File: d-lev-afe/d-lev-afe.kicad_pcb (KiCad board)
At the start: 4 copper layers, 89 x 50 mm, 37 parts, among them J1 S8B-PH-SM4-TB, Q1 MMBT3904, Q2 MMBT3906, U1 74AHC04, U2 AP2112K-3.3, U3 SRV05-4

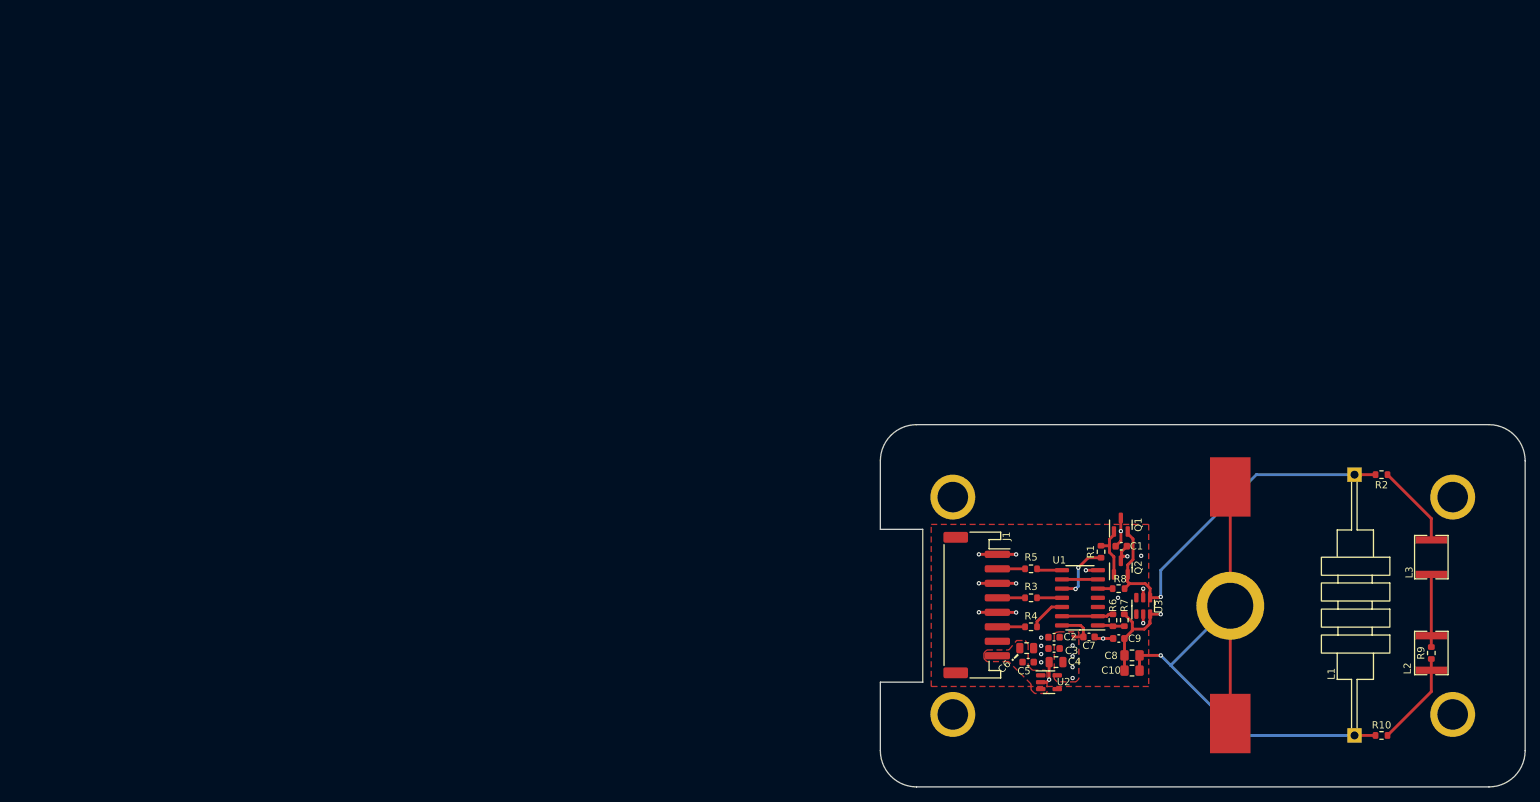
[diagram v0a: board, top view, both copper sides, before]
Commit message: Add JLC releases
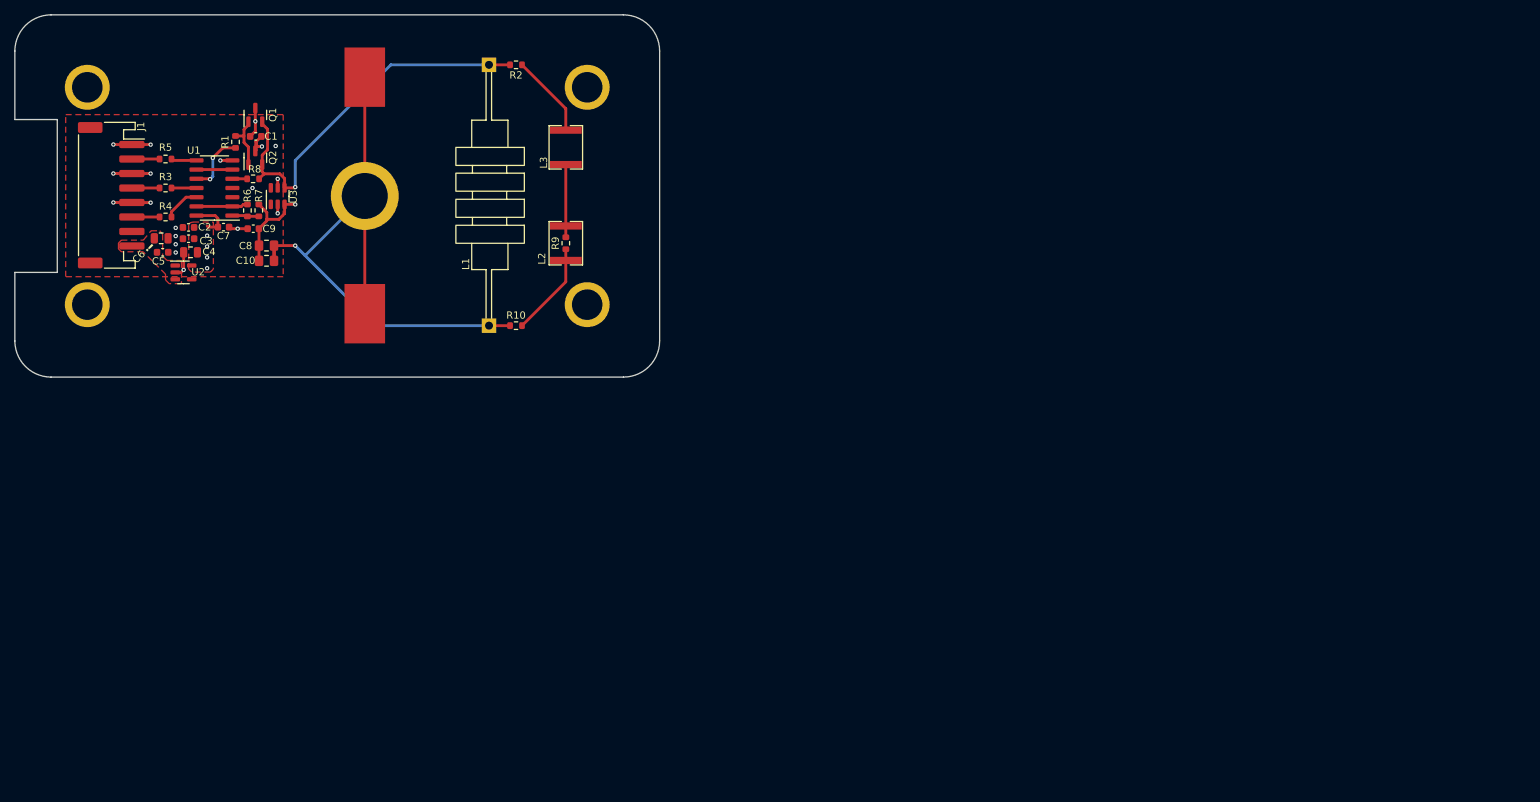
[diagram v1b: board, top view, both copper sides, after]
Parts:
- moved AE1 132.2 mm to (61.8, 25.9)
- moved AE2 132.2 mm to (61.8, 51.0)
- moved C10 132.2 mm to (48.3, 47.5)
- moved C2 132.2 mm to (37.5, 42.9)
- moved C5 132.2 mm to (33.9, 46.3)
- moved C7 132.2 mm to (42.3, 42.8)
- moved C8 132.2 mm to (48.3, 45.4)
- moved G*** 132.2 mm to (92.8, 40.9)
- moved H1 132.2 mm to (23.5, 23.5)
- moved H2 132.2 mm to (92.5, 23.5)
- moved H3 132.2 mm to (23.5, 53.5)
- moved H4 132.2 mm to (61.8, 38.5)
- moved H5 132.2 mm to (92.5, 53.5)
- moved J1 132.2 mm to (26.8, 38.4)
- moved L2 132.2 mm to (89.6, 45.1)
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
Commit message: Add iBOMs and additional part numbers
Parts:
- C1, C7: value 0.1uF -> 100n
- C10: value 1p -> 2.4p
- C2: value .1u -> 100n
- R6: value 220K -> 220k
